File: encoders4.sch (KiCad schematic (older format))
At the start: 29 parts, among them U11 74HCT595, U12 74HC165

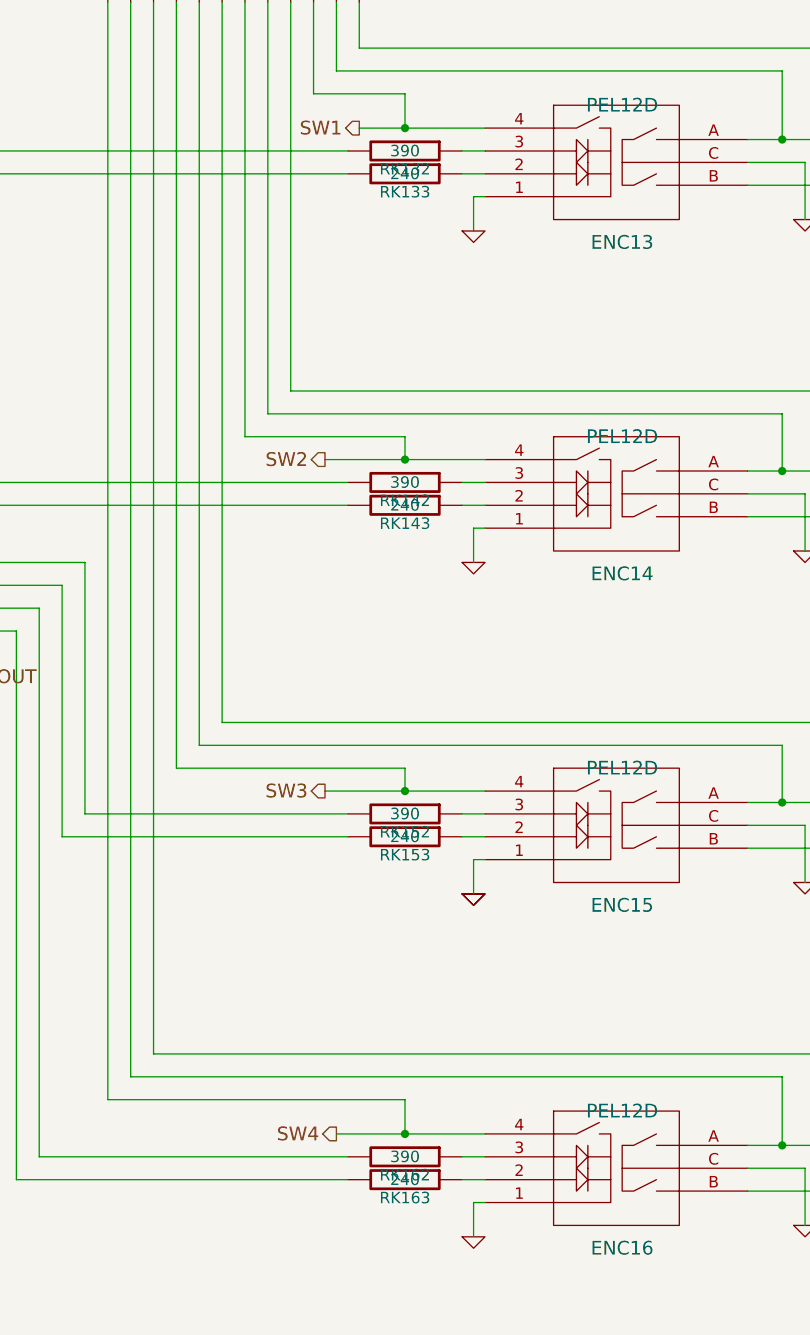
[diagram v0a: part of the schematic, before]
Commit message: Finished board CAD?
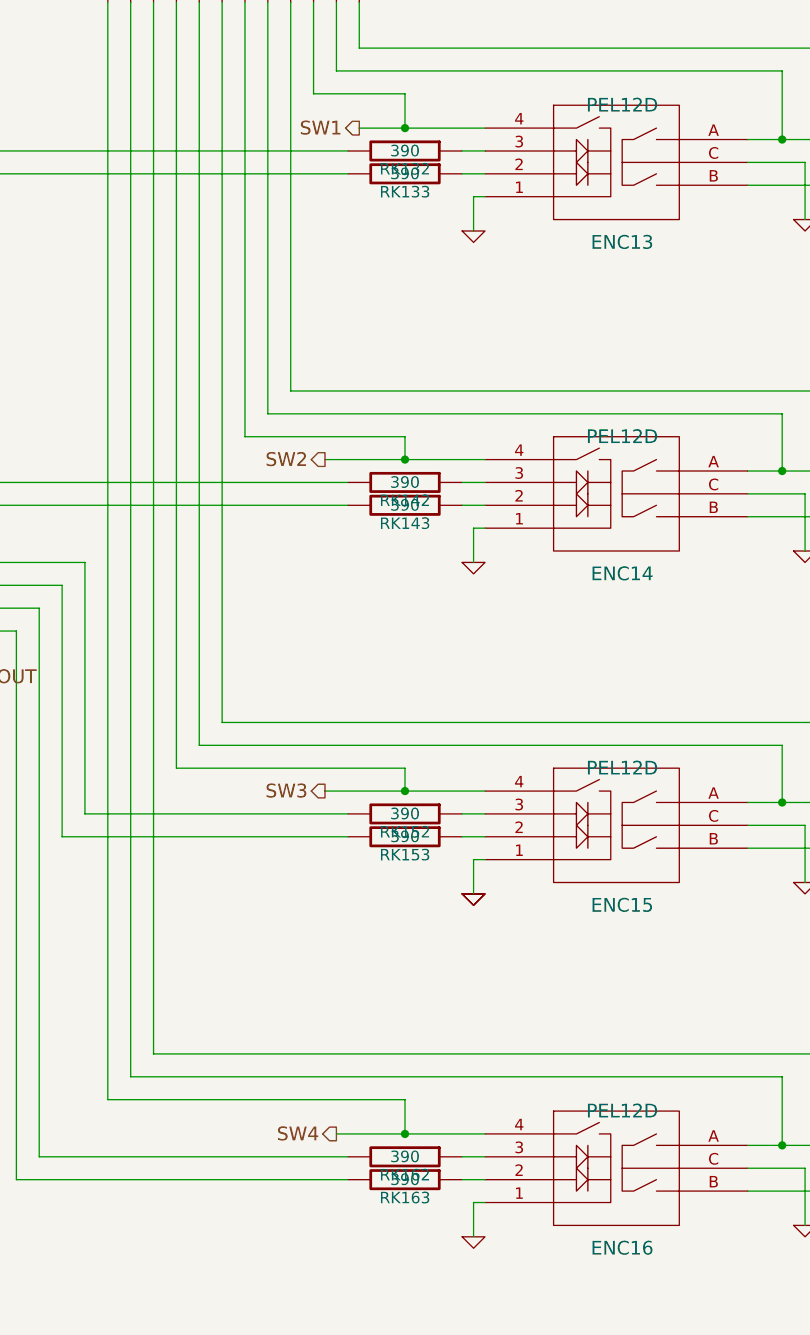
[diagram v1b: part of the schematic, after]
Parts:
- RK133, RK143, RK153, RK163: value 240 -> 390
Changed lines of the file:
@@
-EESchema Schematic File Version 2  date Sat 01 Jun 2013 11:43:44 AM CEST
+EESchema Schematic File Version 2  date Sat 08 Jun 2013 11:15:40 AM CEST
 LIBS:power
 LIBS:device
@@
 Sheet 6 10
 Title ""
-Date "1 jun 2013"
+Date "8 jun 2013"
 Rev ""
 Comp ""
@@
 $EndComp
 $Comp
-L +5V #PWR51
+L +5V #PWR056
 U 1 1 4F92B273
 P 1050 3200
-F 0 "#PWR51" H 1050 3290 20  0001 C CNN
+F 0 "#PWR056" H 1050 3290 20  0001 C CNN
 F 1 "+5V" H 1050 3290 30  0000 C CNN
 	1    1050 3200
@@
 NXP 74HCT595 will source up to 8mA to each output\nand seems to be 5V/3V compatible.
 $Comp
-L +3.3V #PWR66
+L +3.3V #PWR057
 U 1 1 4F92B271
 P 10300 5550
-F 0 "#PWR66" H 10300 5510 30  0001 C CNN
+F 0 "#PWR057" H 10300 5510 30  0001 C CNN
 F 1 "+3.3V" H 10300 5660 30  0000 C CNN
 	1    10300 5550
@@
 $EndComp
 $Comp
-L GND #PWR67
+L GND #PWR058
 U 1 1 4F92B233
 P 10300 6250
-F 0 "#PWR67" H 10300 6250 30  0001 C CNN
+F 0 "#PWR058" H 10300 6250 30  0001 C CNN
 F 1 "GND" H 10300 6180 30  0001 C CNN
 	1    10300 6250
@@
 $EndComp
 $Comp
-L GND #PWR54
+L GND #PWR059
 U 1 1 4F92B231
 P 1850 7150
-F 0 "#PWR54" H 1850 7150 30  0001 C CNN
+F 0 "#PWR059" H 1850 7150 30  0001 C CNN
 F 1 "GND" H 1850 7080 30  0001 C CNN
 	1    1850 7150
@@
 $EndComp
 $Comp
-L +5V #PWR53
+L +5V #PWR060
 U 1 1 4F92B230
 P 1850 6500
-F 0 "#PWR53" H 1850 6590 20  0001 C CNN
+F 0 "#PWR060" H 1850 6590 20  0001 C CNN
 F 1 "+5V" H 1850 6590 30  0000 C CNN
 	1    1850 6500
@@
 $EndComp
 $Comp
-L +3.3V #PWR64
+L +3.3V #PWR061
 U 1 1 4F92B267
 P 9450 3500
-F 0 "#PWR64" H 9450 3460 30  0001 C CNN
+F 0 "#PWR061" H 9450 3460 30  0001 C CNN
 F 1 "+3.3V" H 9450 3610 30  0000 C CNN
 	1    9450 3500
@@
 $EndComp
 $Comp
-L GND #PWR65
+L GND #PWR062
 U 1 1 4F92B265
 P 9450 5250
-F 0 "#PWR65" H 9450 5250 30  0001 C CNN
+F 0 "#PWR062" H 9450 5250 30  0001 C CNN
 F 1 "GND" H 9450 5180 30  0001 C CNN
 	1    9450 5250
@@
 Needs to be 5V/3V compatible --> use HCT
 $Comp
-L GND #PWR52
+L GND #PWR063
 U 1 1 4F92B21B
 P 1050 4700
-F 0 "#PWR52" H 1050 4700 30  0001 C CNN
+F 0 "#PWR063" H 1050 4700 30  0001 C CNN
 F 1 "GND" H 1050 4630 30  0001 C CNN
 	1    1050 4700
@@
 $EndComp
 $Comp
-L GND #PWR58
+L GND #PWR064
 U 1 1 4F92B219
 P 5150 5350
-F 0 "#PWR58" H 5150 5350 30  0001 C CNN
+F 0 "#PWR064" H 5150 5350 30  0001 C CNN
 F 1 "GND" H 5150 5280 30  0001 C CNN
 	1    5150 5350
@@
 $EndComp
 $Comp
-L GND #PWR55
+L GND #PWR065
 U 1 1 4F92B261
 P 5150 2450
-F 0 "#PWR55" H 5150 2450 30  0001 C CNN
+F 0 "#PWR065" H 5150 2450 30  0001 C CNN
 F 1 "GND" H 5150 2380 30  0001 C CNN
 	1    5150 2450
@@
 P 4850 2200
 F 0 "RK133" V 4930 2200 50  0000 C CNN
-F 1 "240" V 4850 2200 50  0000 C CNN
+F 1 "390" V 4850 2200 50  0000 C CNN
 	1    4850 2200
 	0    1    1    0
 $EndComp
 $Comp
-L GND #PWR60
+L GND #PWR066
 U 1 1 4F92B25E
 P 6600 2400
-F 0 "#PWR60" H 6600 2400 30  0001 C CNN
+F 0 "#PWR066" H 6600 2400 30  0001 C CNN
 F 1 "GND" H 6600 2330 30  0001 C CNN
 	1    6600 2400
@@
 $EndComp
 $Comp
-L GND #PWR61
+L GND #PWR067
 U 1 1 4F905A57
 P 6600 3850
-F 0 "#PWR61" H 6600 3850 30  0001 C CNN
+F 0 "#PWR067" H 6600 3850 30  0001 C CNN
 F 1 "GND" H 6600 3780 30  0001 C CNN
 	1    6600 3850
@@
 P 4850 3650
 F 0 "RK143" V 4930 3650 50  0000 C CNN
-F 1 "240" V 4850 3650 50  0000 C CNN
+F 1 "390" V 4850 3650 50  0000 C CNN
 	1    4850 3650
 	0    1    1    0
@@
 $EndComp
 $Comp
-L GND #PWR56
+L GND #PWR068
 U 1 1 4F92B24A
 P 5150 3900
-F 0 "#PWR56" H 5150 3900 30  0001 C CNN
+F 0 "#PWR068" H 5150 3900 30  0001 C CNN
 F 1 "GND" H 5150 3830 30  0001 C CNN
 	1    5150 3900
@@
 $EndComp
 $Comp
-L GND #PWR57
+L GND #PWR069
 U 1 1 4F905A51
 P 5150 5350
-F 0 "#PWR57" H 5150 5350 30  0001 C CNN
+F 0 "#PWR069" H 5150 5350 30  0001 C CNN
 F 1 "GND" H 5150 5280 30  0001 C CNN
 	1    5150 5350
@@
 P 4850 5100
 F 0 "RK153" V 4930 5100 50  0000 C CNN
-F 1 "240" V 4850 5100 50  0000 C CNN
+F 1 "390" V 4850 5100 50  0000 C CNN
 	1    4850 5100
 	0    1    1    0
 $EndComp
 $Comp
-L GND #PWR62
+L GND #PWR070
 U 1 1 4F7E0967
 P 6600 5300
-F 0 "#PWR62" H 6600 5300 30  0001 C CNN
+F 0 "#PWR070" H 6600 5300 30  0001 C CNN
 F 1 "GND" H 6600 5230 30  0001 C CNN
 	1    6600 5300
@@
 $EndComp
 $Comp
-L GND #PWR63
+L GND #PWR071
 U 1 1 4F92B238
 P 6600 6800
-F 0 "#PWR63" H 6600 6800 30  0001 C CNN
+F 0 "#PWR071" H 6600 6800 30  0001 C CNN
 F 1 "GND" H 6600 6730 30  0001 C CNN
 	1    6600 6800
@@
 P 4850 6600
 F 0 "RK163" V 4930 6600 50  0000 C CNN
-F 1 "240" V 4850 6600 50  0000 C CNN
+F 1 "390" V 4850 6600 50  0000 C CNN
 	1    4850 6600
 	0    1    1    0
@@
 $EndComp
 $Comp
-L GND #PWR59
+L GND #PWR072
 U 1 1 4F7E0950
 P 5150 6850
-F 0 "#PWR59" H 5150 6850 30  0001 C CNN
+F 0 "#PWR072" H 5150 6850 30  0001 C CNN
 F 1 "GND" H 5150 6780 30  0001 C CNN
 	1    5150 6850
